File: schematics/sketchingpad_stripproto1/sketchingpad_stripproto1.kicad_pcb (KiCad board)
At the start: 4 copper layers, 158.5 x 66 mm, 83 parts, among them CN1 HC-1.0-4PWT, CN2 S2B-PH-SM4-TB, J3 AudioJack4, Q1 AO3415A, SW1 TC-S3601-3.5-260G-F0.6, SW2 MINI MSK12CO2, U1 TS20, U2 Seeeduino Xiao nRF52840

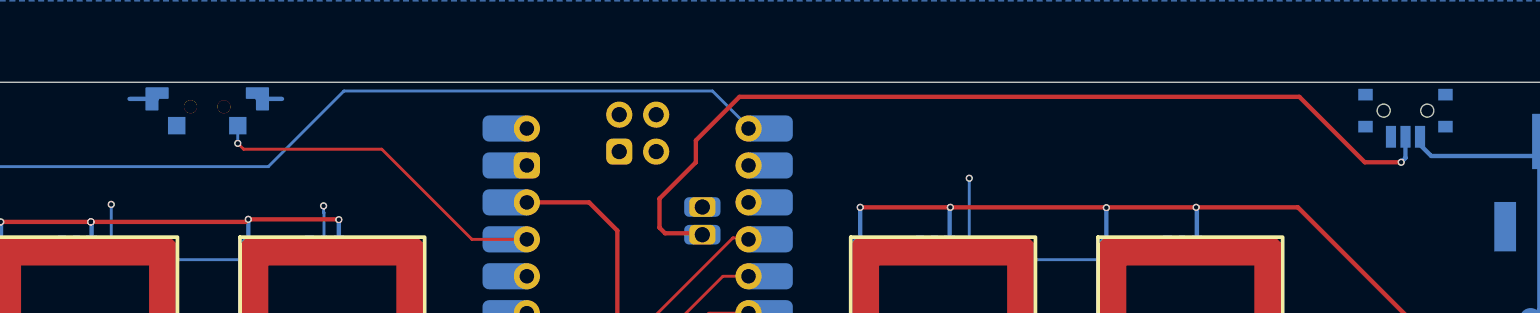
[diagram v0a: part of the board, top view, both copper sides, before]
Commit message: DRC better
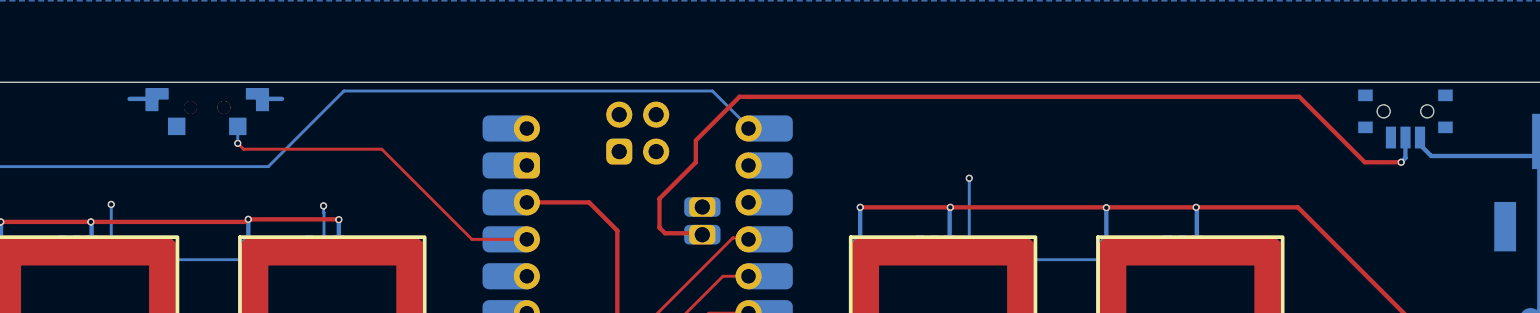
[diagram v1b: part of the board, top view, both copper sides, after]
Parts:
- moved SW2 0.05 mm to (188.8, 62.4)
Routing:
- net 3V3_LED: vias 43 -> 42
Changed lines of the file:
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@@
 	(footprint "easyeda2kicad:SW-SMD_MSK12CO2"
 		(layer "B.Cu")
-		(at 188.795 62.3)
+		(at 188.795 62.35)
 		(property "Reference" "SW2"
 			(at 4.705 -0.3 180)
@@
 	(footprint "easyeda2kicad:SW-SMD_TC-S3601-3.5-260G-F0.6"
 		(layer "B.Cu")
-		(at 106.400051 62.0625 180)
+		(at 106.400051 62.1125 180)
 		(property "Reference" "SW1"
 			(at 0.000051 -2.5375 0)
@@
 		(size 0.5)
 		(drill 0.3)
-		(layers "F.Cu" "B.Cu")
-		(net "3V3_LED")
-	)
-	(via
-		(at 98.4 69.6)
-		(size 0.5)
-		(drill 0.3)
